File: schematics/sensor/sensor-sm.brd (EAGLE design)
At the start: 40 x 25 mm, 22 parts, among them IC1 STM8S208S4, IC2 LP2950CDT-5.0, Q1 8MHz, U1 MCP2551SN

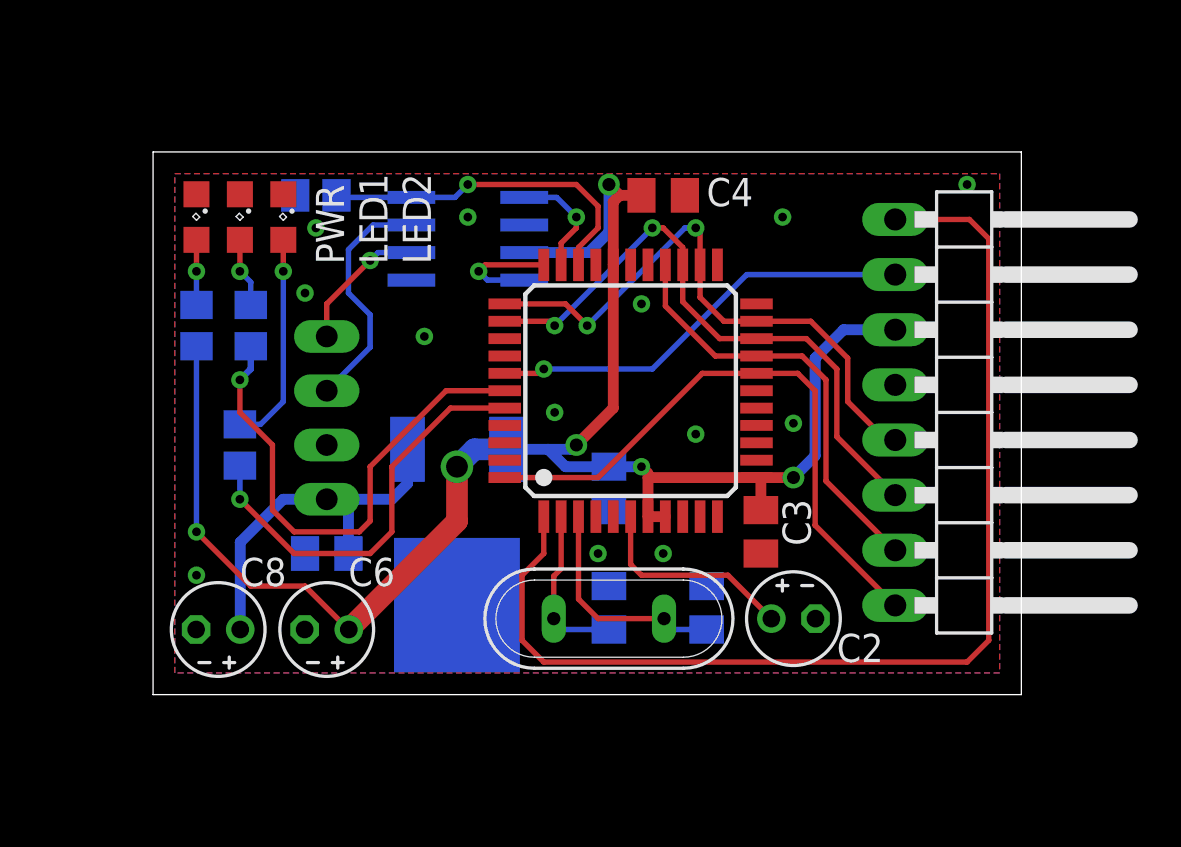
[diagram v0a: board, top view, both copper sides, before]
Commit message: Add latest changes to the home-automation project
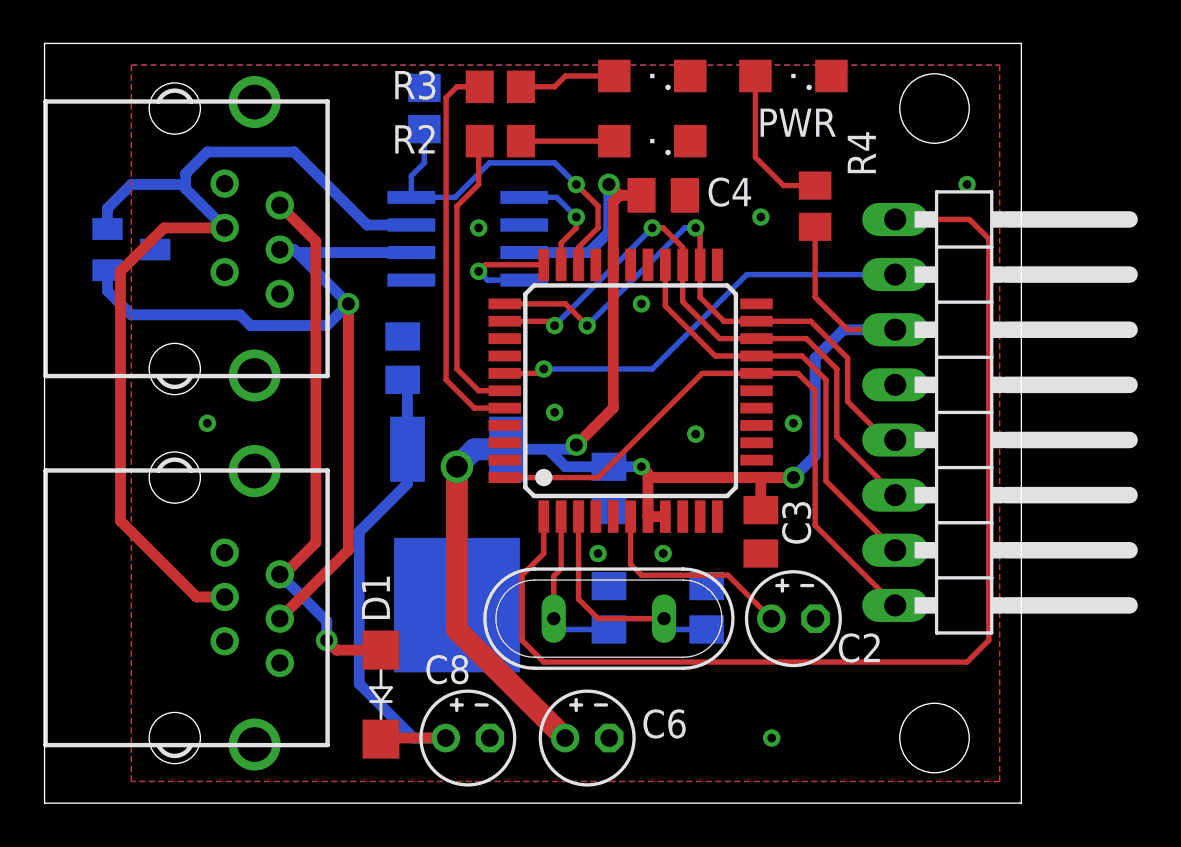
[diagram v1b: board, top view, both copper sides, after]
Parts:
- removed CAN: CWF-4R, connector:CWF-4R
- added D1: GS1J, diode:SMA-DO214AC
- added NUP2105L: NUP2105L, transistor:SOT23
- added X1, X2: YH-55-10, con-wenzhou-yihua:YH-55-10
- LED1, LED2, PWR: device led:SML0805 -> led:SML1206
- moved R4 29.0 mm to (30.5, 22.5), flipped to the top
- moved PWR 28.3 mm to (29.5, 28.5), turned to 180 degrees
- moved R3 20.4 mm to (16.0, 28.0), flipped to the top, turned to 180 degrees
- moved LED1 19.3 mm to (23.0, 25.5), turned to 180 degrees
- moved LED2 18.2 mm to (23.0, 28.5), turned to 180 degrees
- moved R2 14.3 mm to (16.0, 25.5), flipped to the top, turned to 180 degrees
- moved C6 13.0 mm to (20.0, -2.00), turned to 0 degrees
- moved C8 12.5 mm to (14.5, -2.00), turned to 0 degrees
- moved C5 9.66 mm to (11.5, 15.5), turned to 90 degrees
- moved R1 6.40 mm to (12.5, 27.0), turned to 270 degrees
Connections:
- removed net N$2: CAN.P$4, U1.6
- new net N$10: C5.1, C8.+, D1.K, IC2.1
- new net N$9: NUP2105L.2, U1.7, X1.3, X2.3
- net GND: now also NUP2105L.3, X1.5, X2.5; no longer CAN.P$2
- net N$4: now also NUP2105L.1, U1.6, X1.4, X2.4; no longer CAN.P$3, U1.7
- net V_CAN: now also D1.A, X1.2, X2.2; no longer C5.1, C8.+, CAN.P$1, IC2.1
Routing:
- net N$9: track 0.00 -> 43.8 mm
- net N$4: track 11.1 -> 38.4 mm, vias 0 -> 1
- net N$10: track 0.00 -> 23.0 mm
- net LED1: track 23.6 -> 13.5 mm, vias 1 -> 0
- net V_CAN: track 16.9 -> 25.1 mm, vias 0 -> 1
- net N$2: track 6.38 -> 0.00 mm, vias 1 -> 0
- net N$7: track 9.88 -> 4.51 mm, vias 1 -> 0
- net +5V: track 79.7 -> 74.8 mm, vias 6 -> 5
- net N$8: track 3.00 -> 7.04 mm, vias 1 -> 0
- net LED2: track 19.3 -> 18.0 mm, vias 1 -> 0
- net N$6: track 3.21 -> 4.30 mm, vias 1 -> 0
- net CAN_RS: track 15.8 -> 16.6 mm
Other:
- board size 40 x 25 mm -> 45 x 35 mm
- board text added: "1"
- board text added: "2"
- board text added: "HA / CAN NODE 1.2"
- board text removed: "HA / CAN NODE 1.1"
